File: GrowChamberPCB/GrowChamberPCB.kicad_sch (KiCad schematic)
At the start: 78 parts, among them J1 Screw_Terminal_01x02, J11 Conn_01x24_Pin, J3 TYPE-C-31-M-12, J4 Optocoupler to GPIO, J8 To Relay Board, Q1 IRLML6244, Q2 IRLML6244, Q3 IRLML6244, Q4 IRLML6244, Q5 IRLML6244, Q6 IRLML6244, Q7 IRLML6244, SW1 BootMode, SW2 Reset, U1 ESP32-S3-WROOM-1U, U2 MCP1826S, U3 USBLC6-2SC6, U4 TC4428xOA, U5 W25Q128JVS, U6 CR2013-MI2120

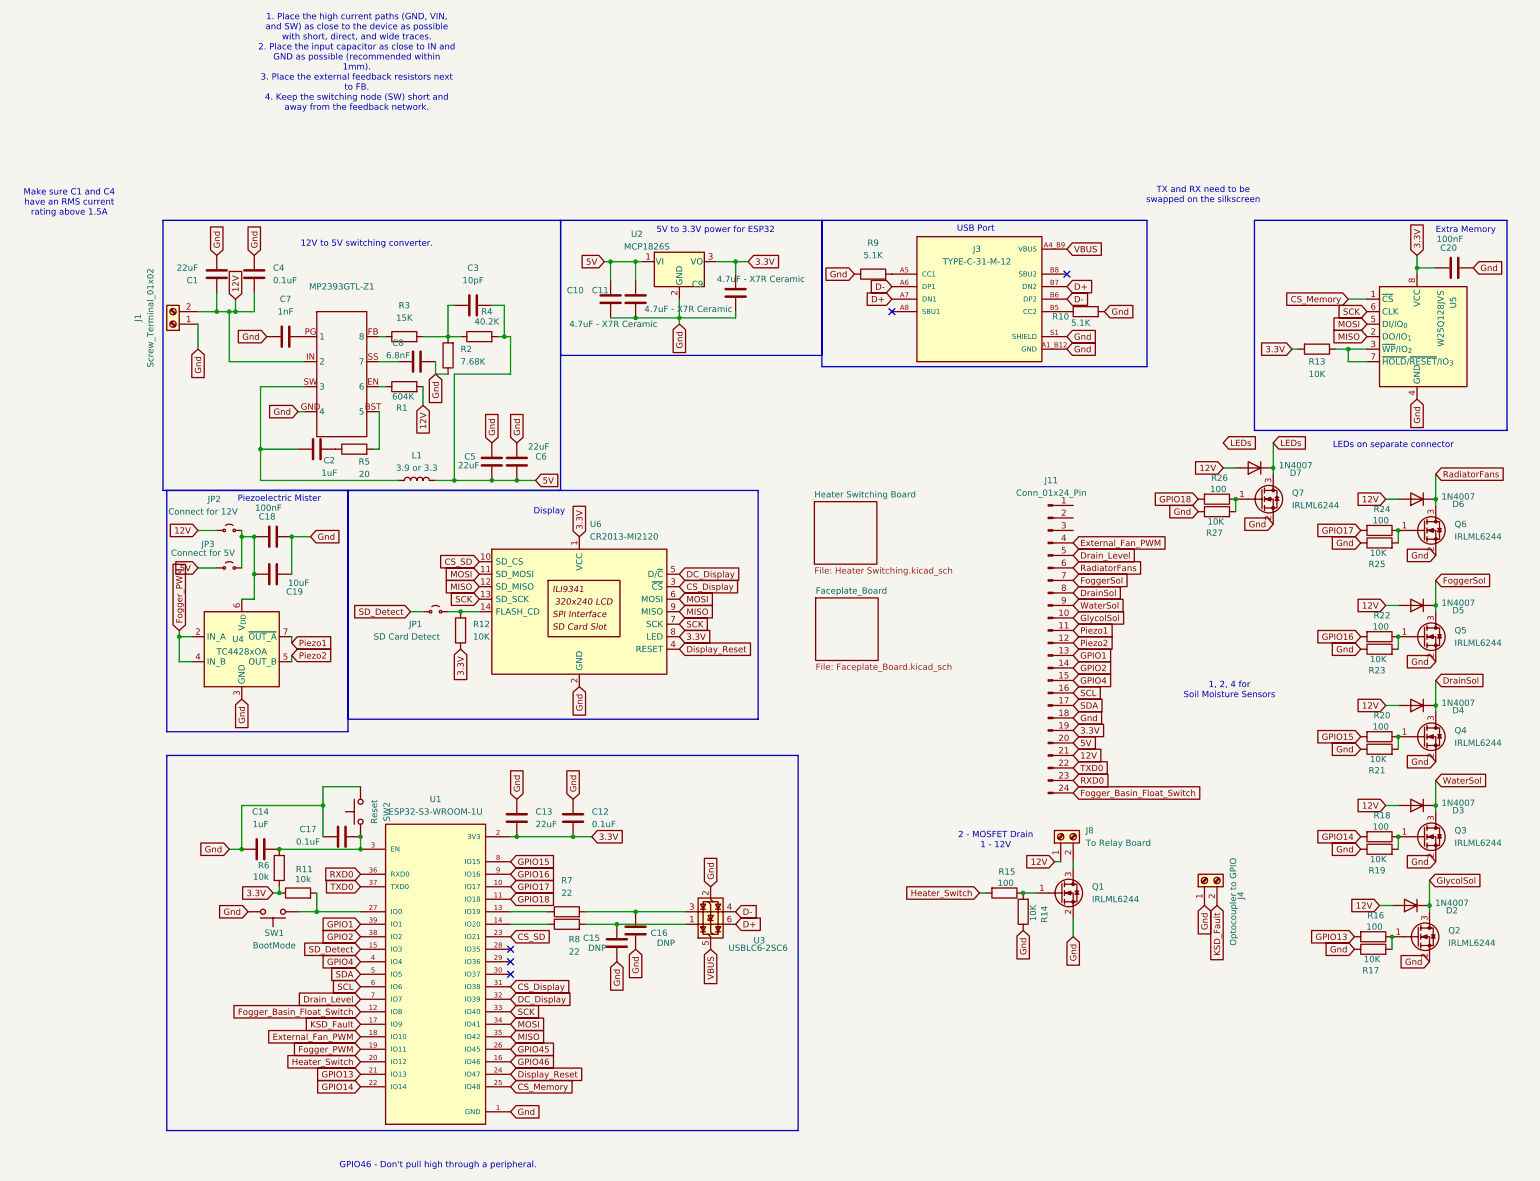
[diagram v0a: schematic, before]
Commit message: Working on faceplate
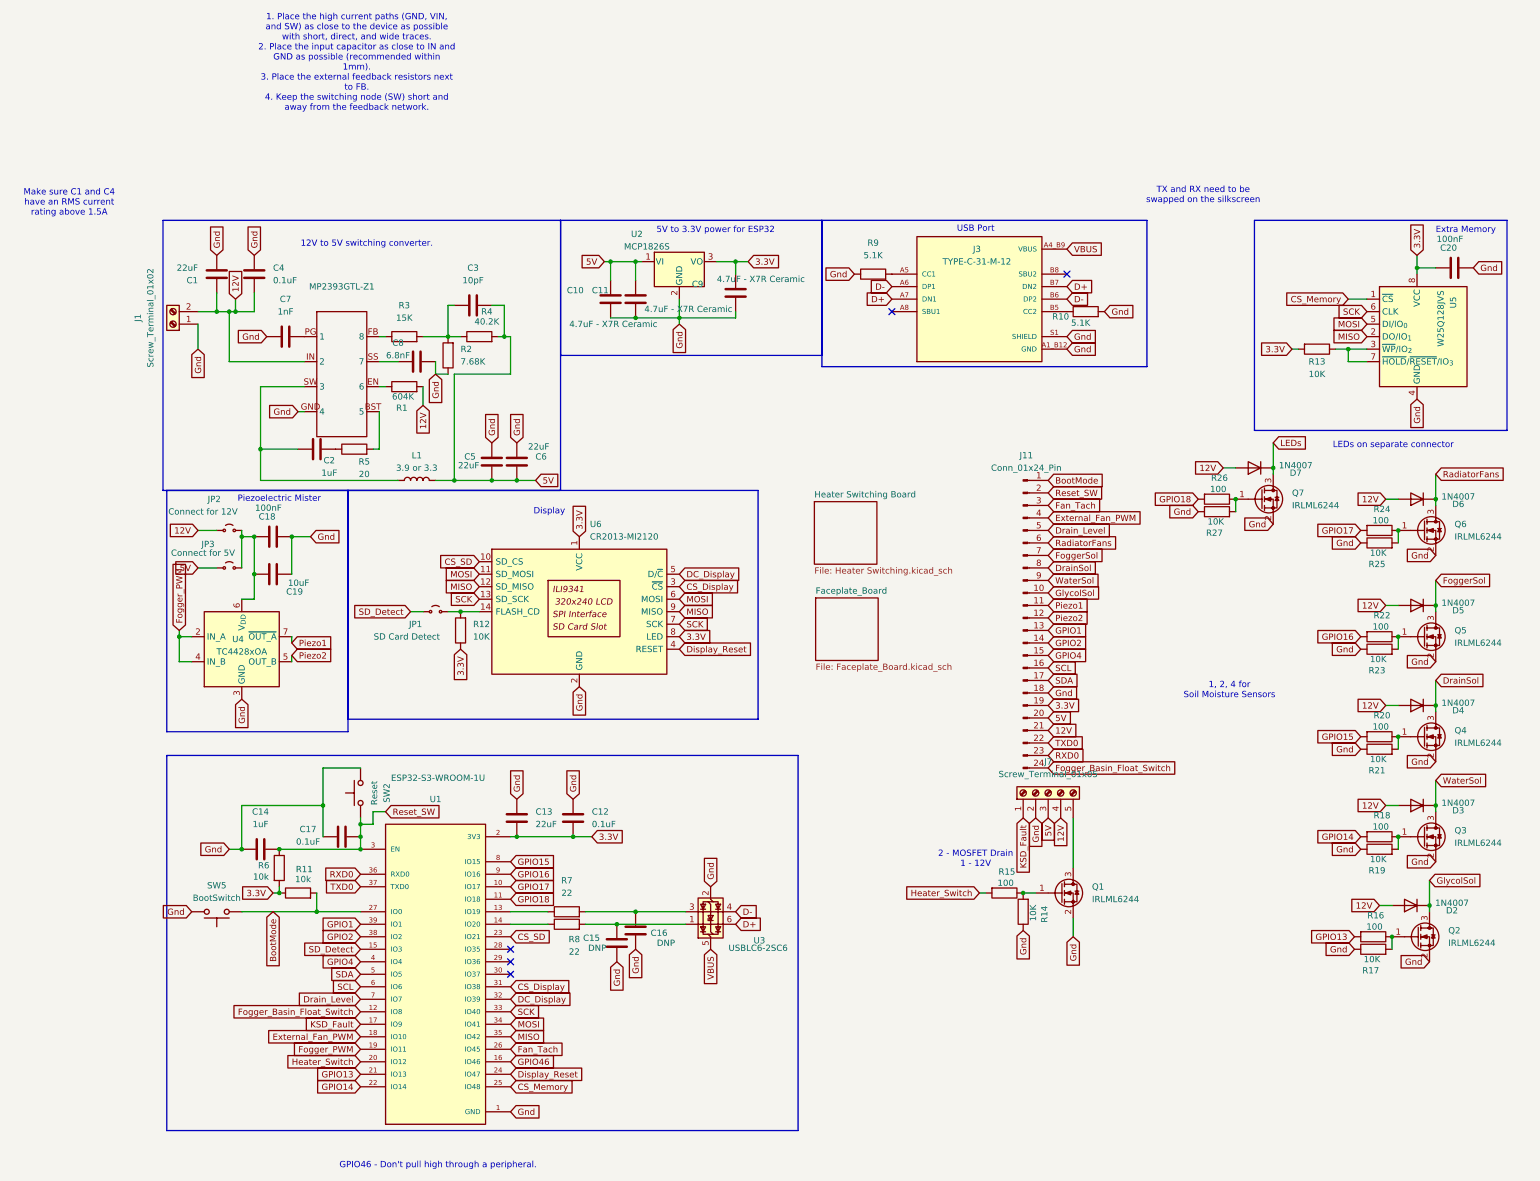
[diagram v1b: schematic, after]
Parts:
- removed J4: Optocoupler to GPIO, symbol Connector:Screw_Terminal_01x02
- removed J8: To Relay Board, symbol Connector:Screw_Terminal_01x02
- removed SW1: BootMode, symbol Switch:SW_Push
- added J7: Screw_Terminal_01x05, symbol Connector:Screw_Terminal_01x05
- added SW5: BootSwitch, symbol Switch:SW_Push
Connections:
- net GPIO45 is gone; now on net Fan_Tach: U1.26 (IO45)
- net 12V: now also J7.4 (Pin_4)
- net 5V: now also J7.3 (Pin_3)
- net GND: now also J7.2 (Pin_2), SW5.2
- net KSD_Fault: now also J7.1 (Pin_1)
- net BootMode: now reaches R11.2, U1.27 (IO0)
- net BootMode: now also J11.1 (Pin_1), SW5.1
- net Reset_SW: now reaches C14.2, C17.2, R6.1, SW2.1, U1.3 (EN)
- net Reset_SW: now also J11.2 (Pin_2)
- net at Q1.3 (D): now also J7.5 (Pin_5)
- net Fan_Tach: now reaches J11.3 (Pin_3)
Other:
- moved on the sheet: J11, SW2

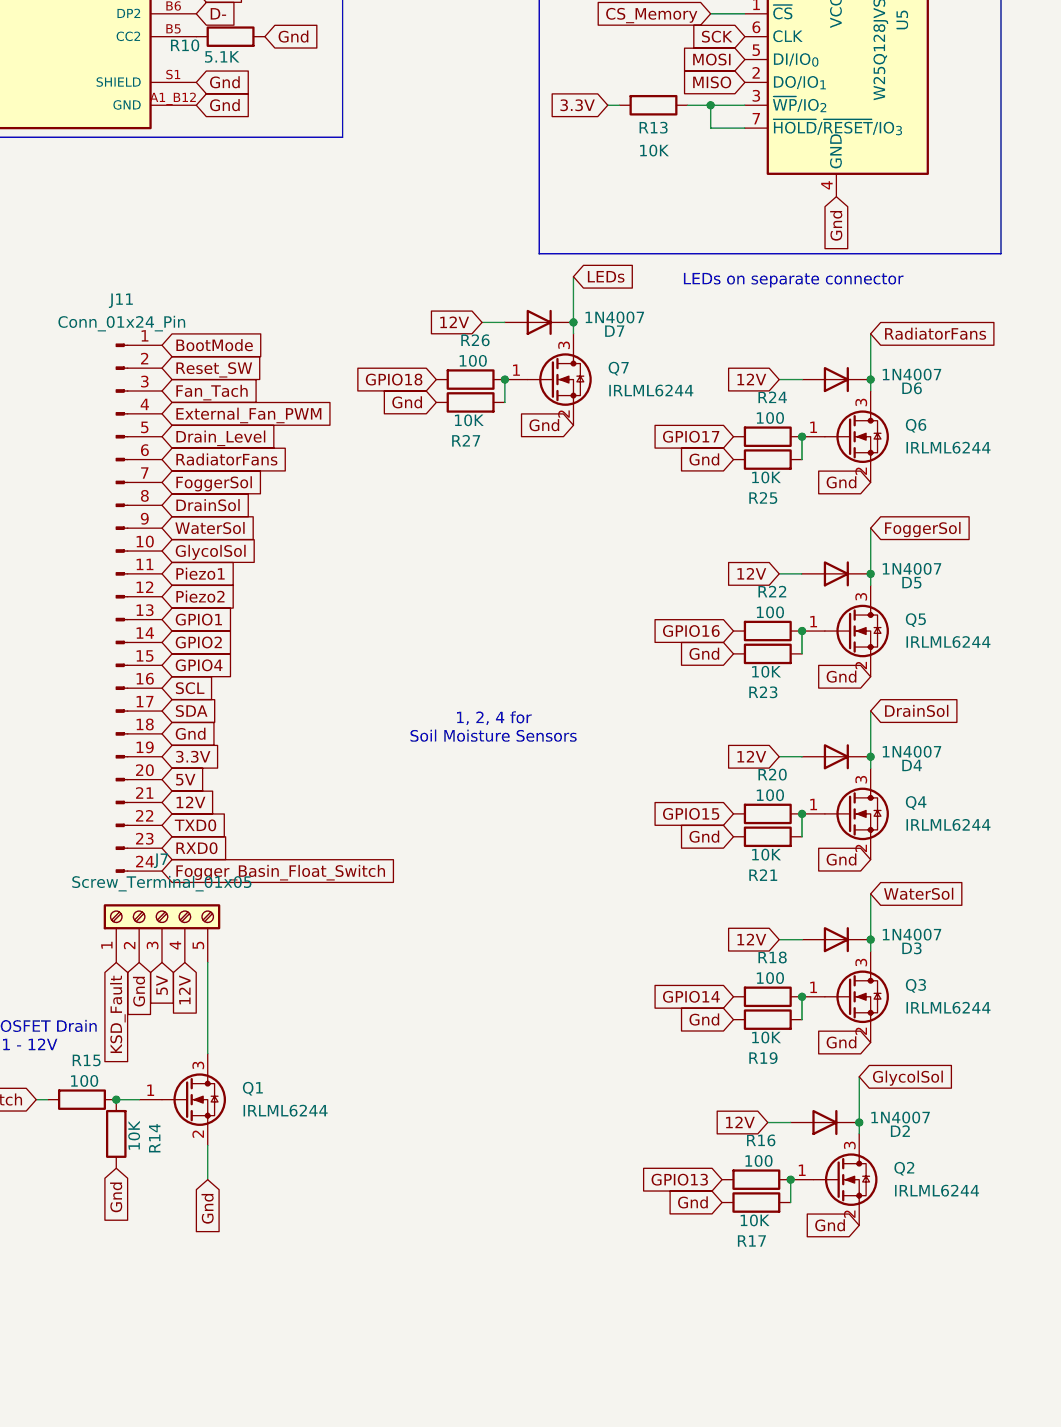
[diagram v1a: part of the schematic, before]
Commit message: final schematic
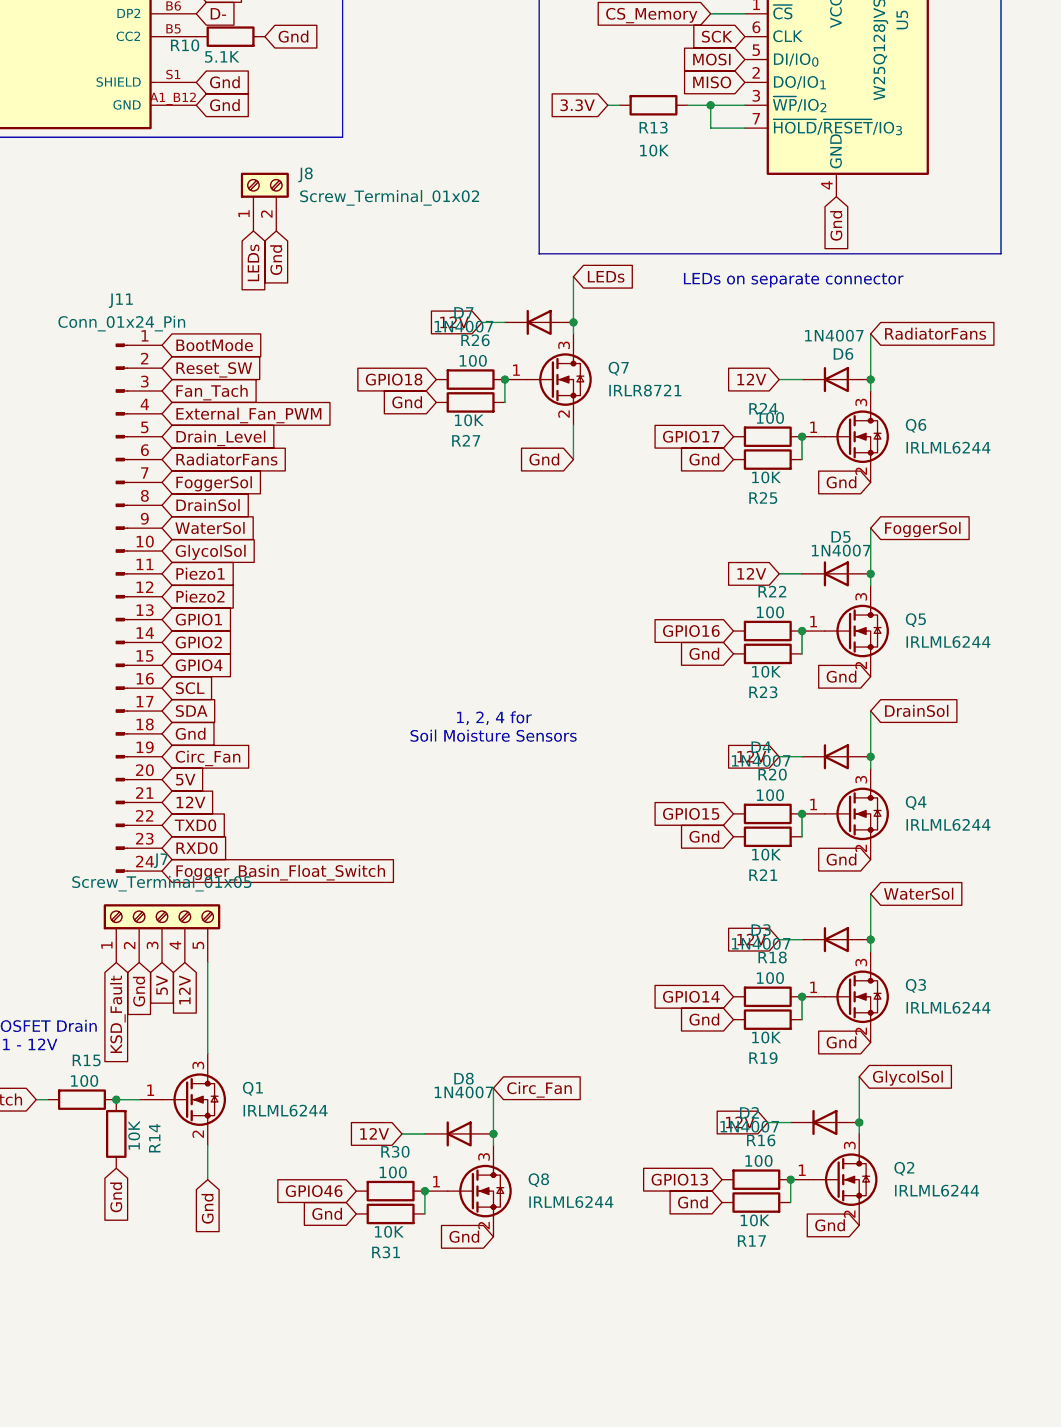
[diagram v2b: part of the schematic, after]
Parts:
- added D8: 1N4007, Diode_SMD:D_SMA, symbol Diode:1N4007
- added J8: Screw_Terminal_01x02, symbol Connector:Screw_Terminal_01x02
- added Q8: IRLML6244, Package_TO_SOT_SMD:SOT-23, symbol Transistor_FET:IRLML6244
- added R30: 100, symbol Device:R
- added R31: 10K, symbol Device:R
- Q7: value IRLML6244 -> IRLR8721; footprint Package_TO_SOT_SMD:SOT-23 -> Package_TO_SOT_SMD:TO-252-2
- U1: footprint ESP32-S3-WROOM-1U:XCVR_ESP32-S3-WROOM-1U -> (none)
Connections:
- net 12V: now also D2.1 (K), D3.1 (K), D4.1 (K), D5.1 (K), D6.1 (K), D7.1 (K), D8.1 (K); no longer D2.2 (A), D3.2 (A), D4.2 (A), D5.2 (A), D6.2 (A), D7.2 (A)
- net 3.3V: no longer J11.19 (Pin_19)
- net DrainSol: now also D4.2 (A); no longer D4.1 (K)
- net FoggerSol: now also D5.2 (A); no longer D5.1 (K)
- net GND: now also J8.2 (Pin_2), Q8.2 (S), R31.1
- net GPIO46: now also R30.2
- net GlycolSol: now also D2.2 (A); no longer D2.1 (K)
- net LEDs: now also D7.2 (A), J8.1 (Pin_1); no longer D7.1 (K)
- net RadiatorFans: now also D6.2 (A); no longer D6.1 (K)
- net WaterSol: now also D3.2 (A); no longer D3.1 (K)
- new net: Q8.1 (G), R30.1, R31.2
- new net Circ_Fan: D8.2 (A), J11.19 (Pin_19), Q8.3 (D)
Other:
- moved on the sheet: D2, D3, D4, D5, D6, D7
